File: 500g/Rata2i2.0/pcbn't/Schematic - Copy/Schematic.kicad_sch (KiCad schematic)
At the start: 43 parts, among them J1 Screw_Terminal_01x03, J10 Conn_01x03_Pin, J11 Screw_Terminal_01x02, J12 Screw_Terminal_01x02, J13 Screw_Terminal_01x03, J14 Screw_Terminal_01x03, J15 Screw_Terminal_01x03, J16 Screw_Terminal_01x07, J2 Screw_Terminal_01x03, J3 Screw_Terminal_01x03, J4 Screw_Terminal_01x03, J5 Screw_Terminal_01x03, J6 Screw_Terminal_01x03, J7 Battery, J8 Conn_01x08_Pin, J9 Screw_Terminal_01x03, SW1 SW_SPDT, U1 DEV-16771, U2 NRF24L01_Breakout, U3 R-78K5.0-0.5, U4 R-78K5.0-0.5, U5 DRV8871DDAR

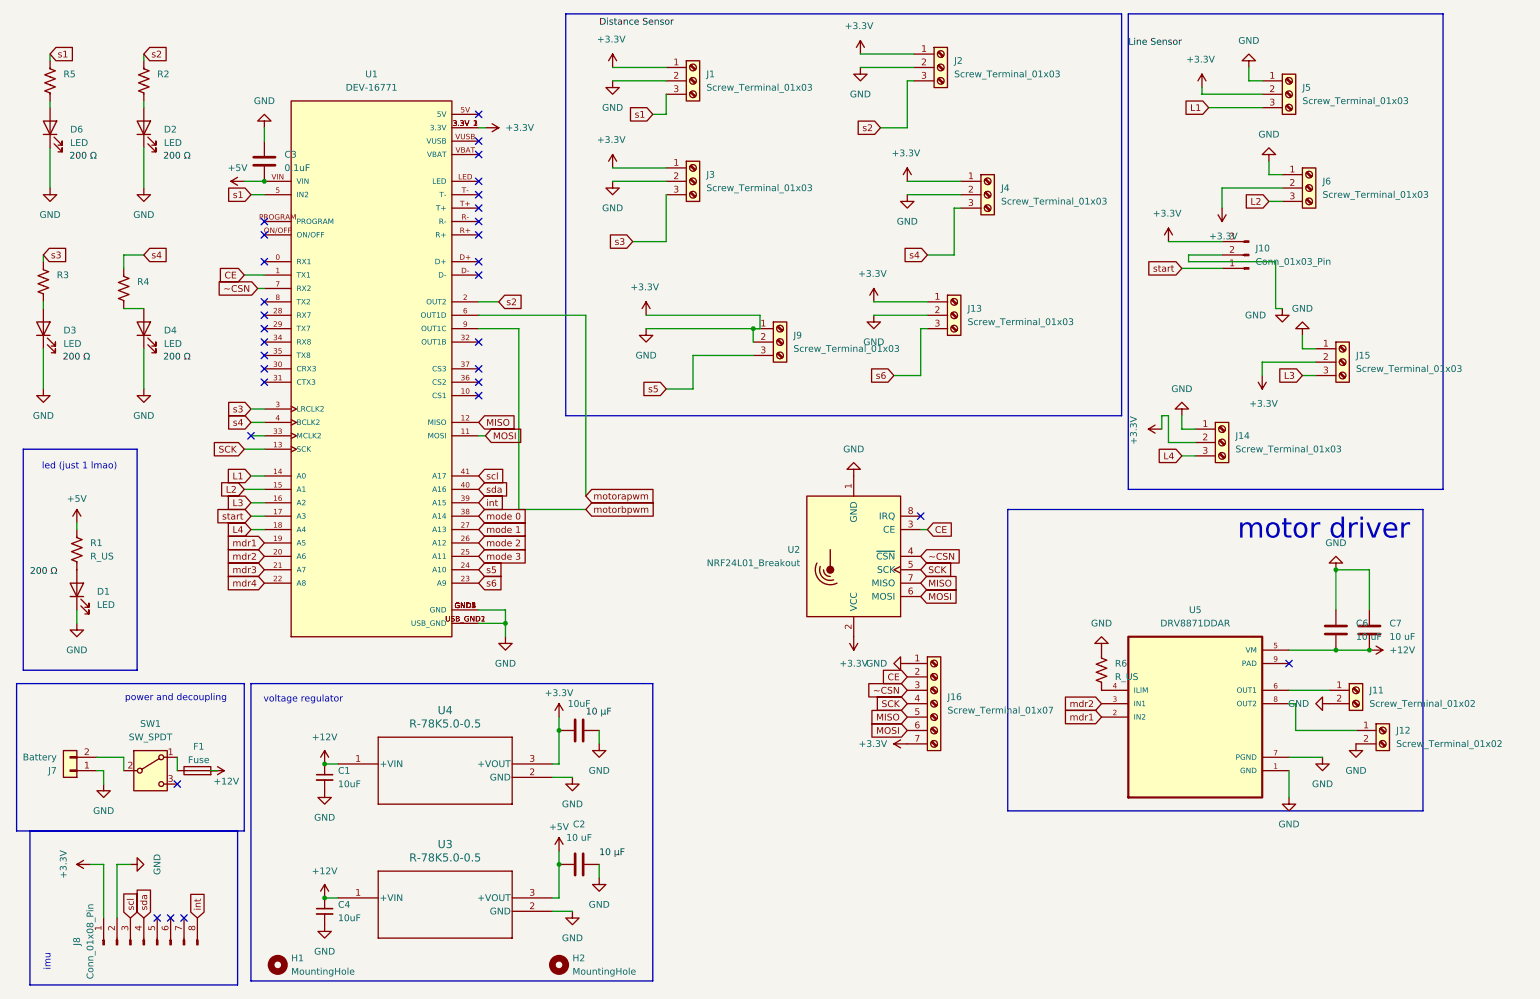
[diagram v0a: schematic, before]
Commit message: 2 motor drivers, 2 less sensors :D
mostly connected but it REALLY doesn't like the motor drivers, maybe moving to the normal side will make it better?
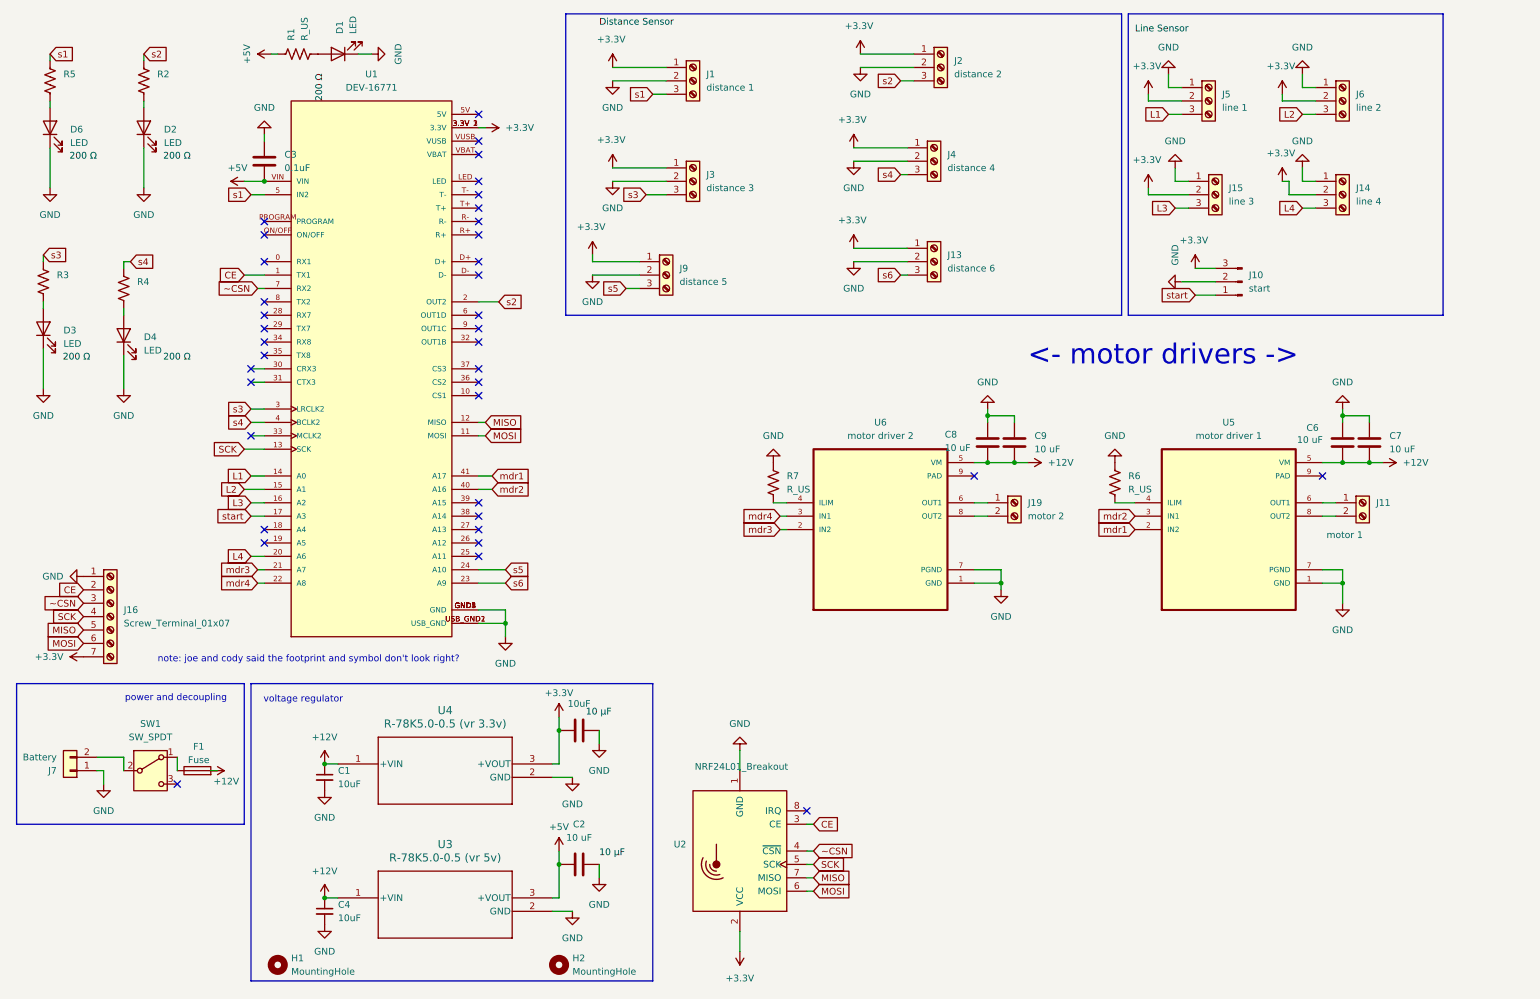
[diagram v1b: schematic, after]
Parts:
- removed J12: Screw_Terminal_01x02, TerminalBlock:TerminalBlock_Xinya_XY308-2.54-2P_1x02_P2.54mm_Horizontal, symbol Connector:Screw_Terminal_01x02
- removed J8: Conn_01x08_Pin, Connector_PinHeader_2.54mm:PinHeader_1x08_P2.54mm_Vertical, symbol Connector:Conn_01x08_Pin
- added C8, C9: 10 uF, Capacitor_SMD:C_0805_2012Metric, symbol Device:C
- added J19: motor 2, TerminalBlock:TerminalBlock_Xinya_XY308-2.54-2P_1x02_P2.54mm_Horizontal, symbol Connector:Screw_Terminal_01x02
- added R7: R_US, Resistor_SMD:R_0805_2012Metric, symbol Device:R_US
- added U6: motor driver 2, DRV8871DDAR:VREG_LM5017MR_NOPB, symbol DRV8871DDAR:DRV8871DDAR
- J1: value Screw_Terminal_01x03 -> distance 1
- J10: value Conn_01x03_Pin -> start; footprint Connector_PinHeader_2.54mm:PinHeader_1x03_P2.54mm_Vertical -> TerminalBlock:TerminalBlock_Xinya_XY308-2.54-3P_1x03_P2.54mm_Horizontal
- J11: value Screw_Terminal_01x02 -> motor 1
- J13: value Screw_Terminal_01x03 -> distance 6
- J14: value Screw_Terminal_01x03 -> line 4
- J15: value Screw_Terminal_01x03 -> line 3
- J2: value Screw_Terminal_01x03 -> distance 2
- J3: value Screw_Terminal_01x03 -> distance 3
- J4: value Screw_Terminal_01x03 -> distance 4
- J5: value Screw_Terminal_01x03 -> line 1
- J6: value Screw_Terminal_01x03 -> line 2
- J9: value Screw_Terminal_01x03 -> distance 5
- U3: value R-78K5.0-0.5 -> R-78K5.0-0.5 (vr 5v)
- U4: value R-78K5.0-0.5 -> R-78K5.0-0.5 (vr 3.3v)
- U5: value DRV8871DDAR -> motor driver 1
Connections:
- net scl is gone; now on net mdr1: U1.41 (A17)
- net sda is gone; now on net mdr2: U1.40 (A16)
- net +12V: now also C8.1, C9.1, U6.5 (VM)
- net +3.3V: no longer C1.2, C2.2, C3.1, C4.2, C5.2, C6.2, C7.2, D1.1 (K), D2.1 (K), D3.1 (K), D4.1 (K), D6.1 (K), J1.2 (Pin_2), J10.2 (Pin_2), J11.2 (Pin_2), J13.2 (Pin_2), J14.1 (Pin_1), J15.1 (Pin_1), J16.1 (Pin_1), J2.2 (Pin_2), J3.2 (Pin_2), J4.2 (Pin_2), J5.1 (Pin_1), J6.1 (Pin_1), J7.1 (Pin_1), J9.2 (Pin_2), R6.1, U1.GND1 (GND), U1.GND2 (GND), U1.GND3 (GND), U1.GND4 (GND), U1.GND5 (GND), U1.USB_GND1 (USB_GND), U1.USB_GND2 (USB_GND), U2.1 (GND), U3.2 (GND), U4.2 (GND), U5.1 (GND), U5.7 (PGND)
- net L4: now also U1.20 (A6); no longer U1.18 (A4)
- net mdr1: no longer U1.19 (A5)
- net mdr2: no longer U1.20 (A6)
- net mdr3: now also U6.2 (IN2)
- net mdr4: now also U6.3 (IN1)
- net at U5.8 (OUT2): now also J11.2 (Pin_2)
- net int: no longer names the net of U1.39 (A15)
- net mode 0: no longer names the net of U1.38 (A14)
- net mode 1: no longer names the net of U1.27 (A13)
- net mode 2: no longer names the net of U1.26 (A12)
- net mode 3: no longer names the net of U1.25 (A11)
- net motorapwm: no longer names the net of U1.6 (OUT1D)
- net motorbpwm: no longer names the net of U1.9 (OUT1C)
- new net: R7.2, U6.4 (ILIM)
- new net: J19.1 (Pin_1), U6.6 (OUT1)
- new net: J19.2 (Pin_2), U6.8 (OUT2)
- new net GND: C1.2, C2.2, C3.1, C4.2, C5.2, C6.2, C7.2, C8.2, C9.2, D1.1 (K), D2.1 (K), D3.1 (K), D4.1 (K), D6.1 (K), J1.2 (Pin_2), J10.2 (Pin_2), J13.2 (Pin_2), J14.1 (Pin_1), J15.1 (Pin_1), J16.1 (Pin_1), J2.2 (Pin_2), J3.2 (Pin_2), J4.2 (Pin_2), J5.1 (Pin_1), J6.1 (Pin_1), J7.1 (Pin_1), J9.2 (Pin_2), R6.1, R7.1, U1.GND1 (GND), U1.GND2 (GND), U1.GND3 (GND), U1.GND4 (GND), U1.GND5 (GND), U1.USB_GND1 (USB_GND), U1.USB_GND2 (USB_GND), U2.1 (GND), U3.2 (GND), U4.2 (GND), U5.1 (GND), U5.7 (PGND), U6.1 (GND), U6.7 (PGND)
- no-connect marks 31 -> 38
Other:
- note added: "<- motor drivers ->"
- note added: "note: joe and cody said the footprint and symbol don't look right?"
- note removed: "imu"
- note removed: "led (just 1 lmao)"
- note removed: "motor driver"
- moved on the sheet: C6, C7, D1, D4, J10, J11, J13, J14, J15, J16, J4, J5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
